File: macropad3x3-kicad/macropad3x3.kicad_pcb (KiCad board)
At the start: 2 copper layers, 77 x 112.5 mm, 26 parts, among them J1 OLED-4PIN, U1 Arduino_Pro_Micro

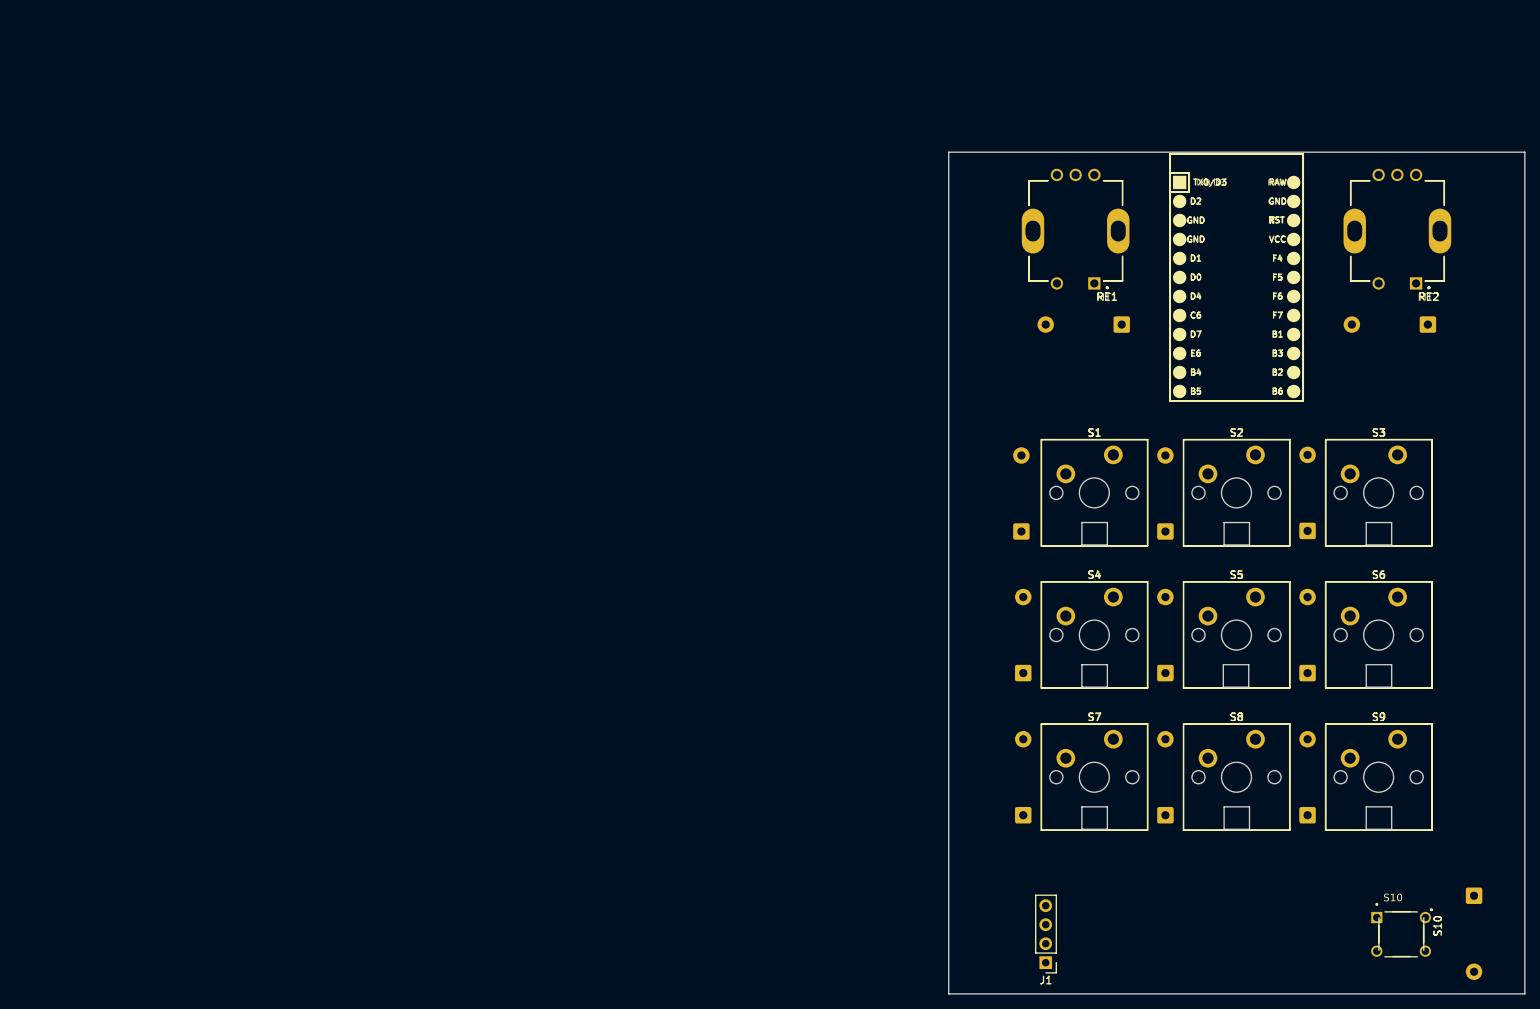
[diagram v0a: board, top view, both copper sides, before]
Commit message: hi
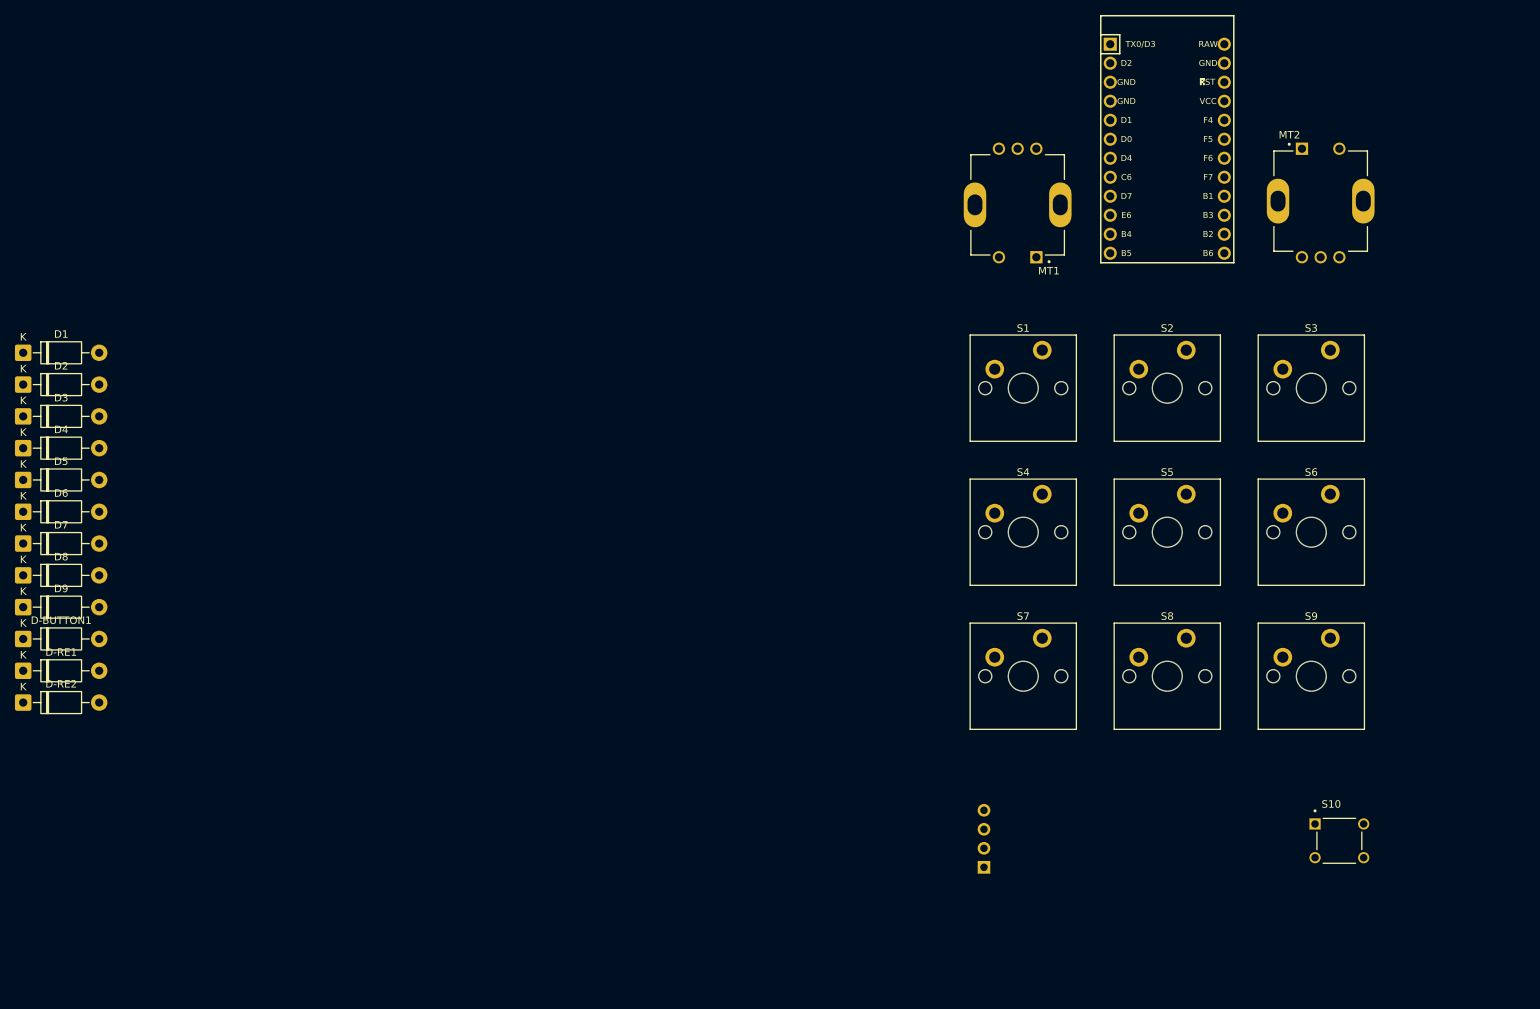
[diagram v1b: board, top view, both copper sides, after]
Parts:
- D-BUTTON1, D-RE1, D-RE2, D1, D2, D3, D4, D5, D6, D7, D8, D9: moved to F.Cu
- moved D-BUTTON1 196.9 mm to (-31.2, 115.8), turned to 0 degrees
- moved D-RE2 194.4 mm to (-31.2, 124.3), turned to 0 degrees
- moved D9 173.9 mm to (-31.2, 111.5), turned to 0 degrees
- moved D6 173.0 mm to (-31.2, 98.8), turned to 0 degrees
- moved D3 172.3 mm to (-31.2, 86.0), turned to 0 degrees
- moved D8 156.0 mm to (-31.2, 107.3), turned to 0 degrees
- moved D5 154.8 mm to (-31.2, 94.5), turned to 0 degrees
- moved D-RE1 153.9 mm to (-31.2, 120.0), turned to 0 degrees
- moved D2 153.9 mm to (-31.2, 81.8), turned to 0 degrees
- moved D7 138.5 mm to (-31.2, 103.0), turned to 0 degrees
- moved D4 137.0 mm to (-31.2, 90.3), turned to 0 degrees
- moved D1 135.5 mm to (-31.2, 77.5), turned to 0 degrees
- moved U1 20.7 mm to (121.8, 50.2)
- moved S1 16.9 mm to (102.5, 82.2)
- moved S2 16.8 mm to (121.8, 82.2)
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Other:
- board outline removed
